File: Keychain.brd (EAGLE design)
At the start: 86 x 54 mm, 12 parts, among them IC1 LM555D, J1 UX60-MB-5S8, Q2 BSS806N, SW1 MFS101D-6-Z

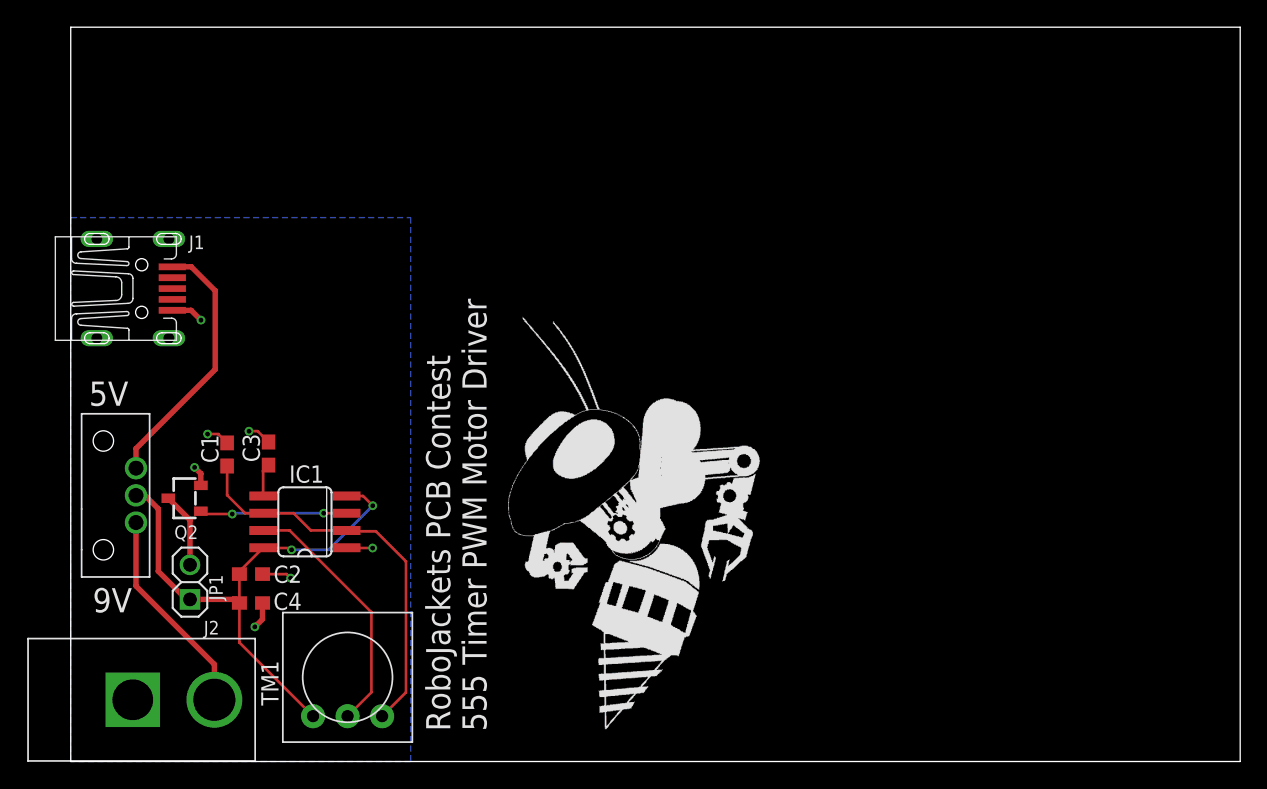
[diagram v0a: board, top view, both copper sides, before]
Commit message: Made a thing
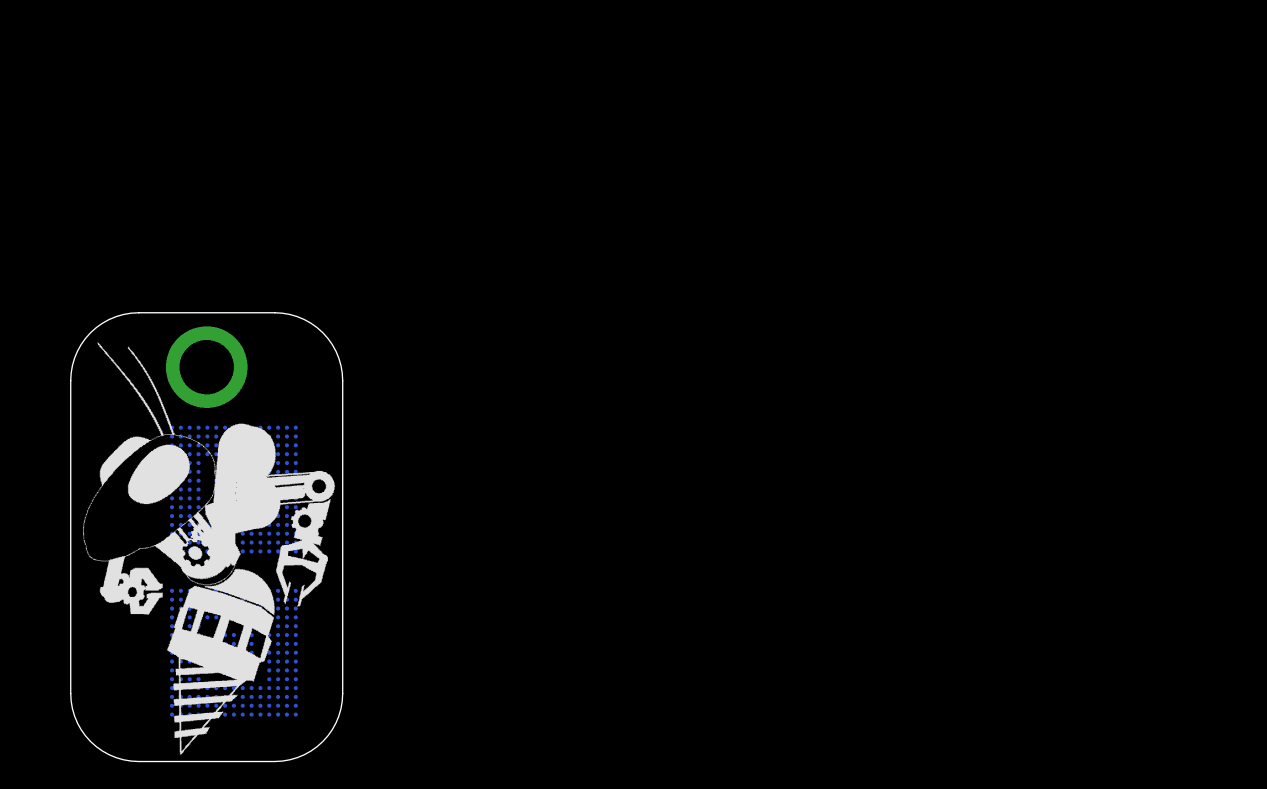
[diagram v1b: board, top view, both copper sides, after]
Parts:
- removed C1, C3: 0.01uF, rcl:C0603
- removed C2: 0.1uF, rcl:C0603
- removed C4: 10uF, rcl:C0603
- removed IC1: LM555D, adafruit:SO08
- removed J1: UX60-MB-5S8, RoboJackets-Connectors:UX60-MB-5S8
- removed J2: (no value), RoboJackets-Connectors:PJ-037A
- removed JP1: (no value), RoboJackets-Connectors:1X02
- removed Q2: BSS806N, RoboJackets-Discrete:SOT-23-3
- removed SW1: MFS101D-6-Z, Example:MFS101D-6-Z
- removed TM1: (no value), adafruit:TRIM-3386
- removed U$2: (no value), RoboJackets-Aesthetics:ROBOBUZZ_1.4X
- added U1, U2: (no value), mTrain:UFBGA176+25
- added U3: (no value), RoboJackets-Aesthetics:ROBOJACKETS
- added U4: (no value), RoboJackets-Aesthetics:ROBOBUZZ_1.4X
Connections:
- removed net +9V: C2.1, C4.1, IC1.4, IC1.8, JP1.1, SW1.2, TM1.1
- removed net GND: C1.2, C2.2, C3.2, C4.2, IC1.1, J1.5, J2.P$1, Q2.2
- removed net N$1: IC1.7, TM1.2
- removed net N$2: JP1.2, Q2.3
- removed net N$3: C3.1, IC1.5
- removed net N$4: J1.1, SW1.3
- removed net N$6: J2.P$2, SW1.1
- removed net THR: C1.1, IC1.2, IC1.6, TM1.3
- removed net T_OUT: IC1.3, Q2.1
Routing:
- net +9V: track 40.6 -> 0.00 mm, vias 2 -> 0
- net THR: track 29.4 -> 0.00 mm
- net N$4: track 19.3 -> 0.00 mm
- net N$1: track 18.8 -> 0.00 mm, vias 0 -> 1
- net N$6: track 15.4 -> 0.00 mm
- net GND: track 13.5 -> 0.00 mm, vias 7 -> 0
- net T_OUT: track 10.8 -> 0.00 mm, vias 2 -> 0
- net N$2: track 5.56 -> 0.00 mm
- net N$3: track 2.43 -> 0.00 mm
- removed copper zone on layer 16, net GND
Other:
- board size 86 x 54 mm -> 20 x 33 mm
- board text removed: "5V"
- board text removed: "9V"
- board text removed: "RoboJackets PCB Contest 555 Timer PWM Motor Driver"
